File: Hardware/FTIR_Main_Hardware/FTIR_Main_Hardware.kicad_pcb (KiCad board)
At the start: 2 copper layers, 72.3 x 35.1 mm, 77 parts, among them J1 RJ45_LED_Shielded, Q1 IRF7606PBF, Q2 BSS138, Q3 IRF7606PBF, Q4 IRF7606PBF, Q5 BSS138, Q6 BSS138, U1 Opamp_Dual, U2 D36V28F7, U3 OKI, U4 TMC2208_Breakout, U6 Teensy4.1_DEV-16771, U7 OKI

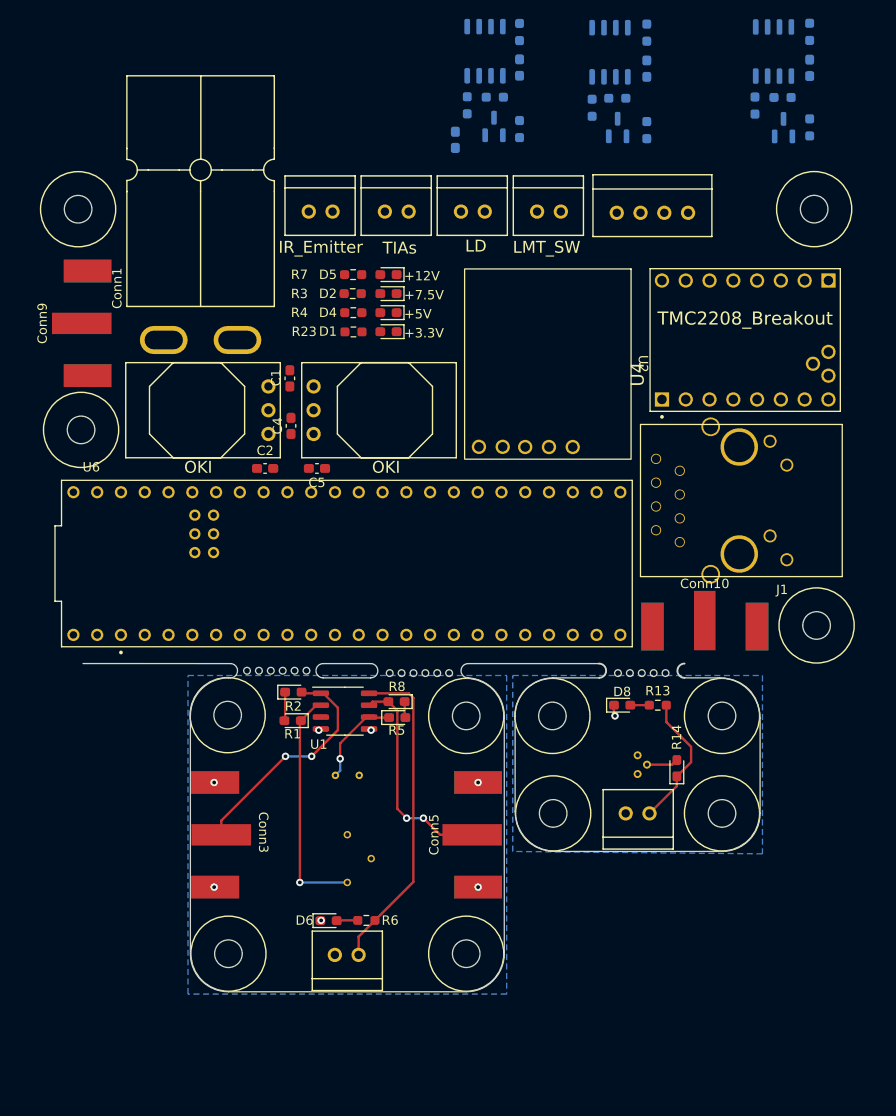
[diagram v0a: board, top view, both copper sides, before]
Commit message: Edge cuts and placing
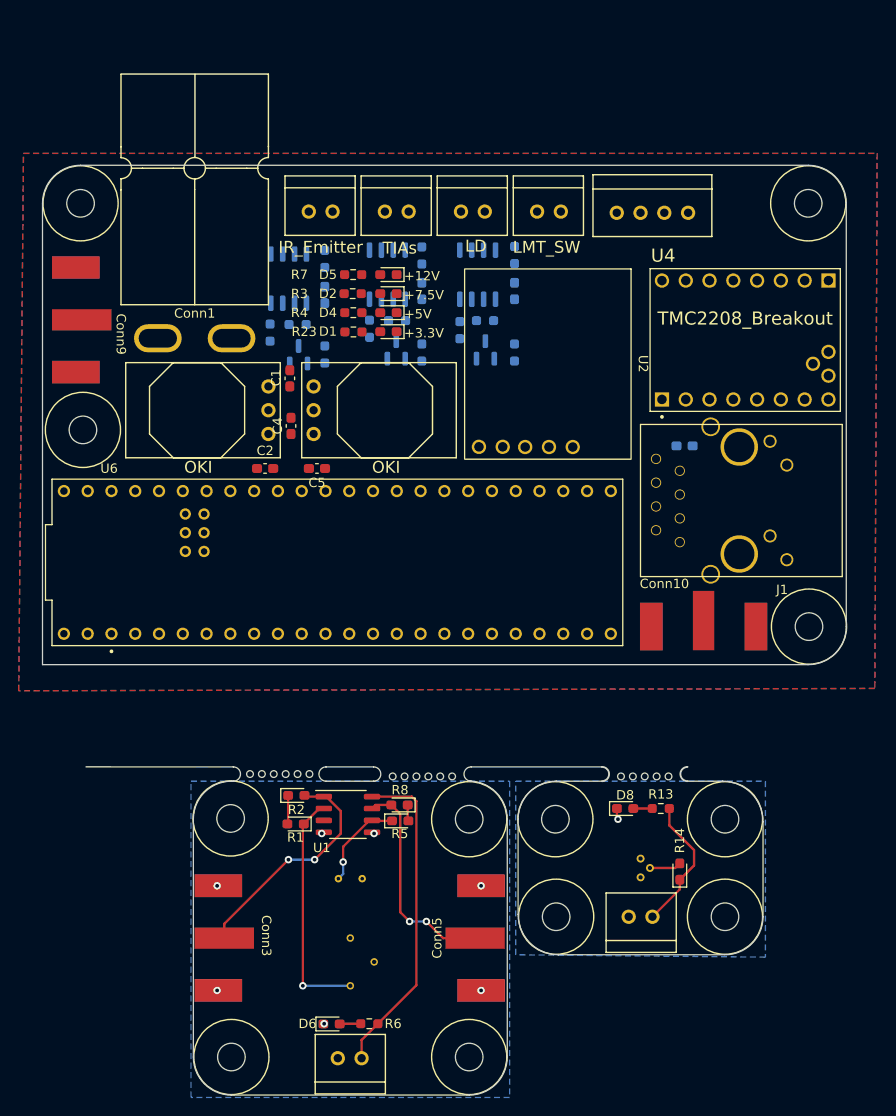
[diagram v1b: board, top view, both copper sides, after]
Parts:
- moved R10 57.2 mm to (128.1, 76.2)
- moved Q1 57.2 mm to (127.1, 71.3)
- moved R11 57.2 mm to (125.1, 77.1)
- moved D7 57.2 mm to (131.0, 73.0)
- moved Q2 57.2 mm to (128.2, 79.4)
- moved R12 57.2 mm to (131.0, 79.4)
- moved R9 57.2 mm to (131.0, 69.2)
- moved C3 40.8 mm to (169.4, 89.2), turned to 180 degrees
- moved R18 27.6 mm to (145.4, 76.8)
- moved Q4 27.6 mm to (147.3, 70.9)
- moved R20 27.6 mm to (151.3, 68.8)
- moved R22 27.6 mm to (151.3, 79.2)
- moved D10 27.6 mm to (151.3, 72.6)
- moved R16 27.6 mm to (148.1, 75.8)
- moved Q6 27.6 mm to (148.1, 78.9)
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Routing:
- added copper zone on F.Cu, net GND
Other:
- board size 72.3 x 35.1 mm -> 85.9 x 99.3 mm
